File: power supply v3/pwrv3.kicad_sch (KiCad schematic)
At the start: 55 parts, among them IC1 TLV3701IDBVR, IC2 LM25145RGYR, IC3 LMR50410YQDBVRQ1, J1 1.5 mm, J3 1933189, J4 Conn_01x04_Pin 1.27mm, Q1 35A, 30V, Q2 35A Id, 30V Vds

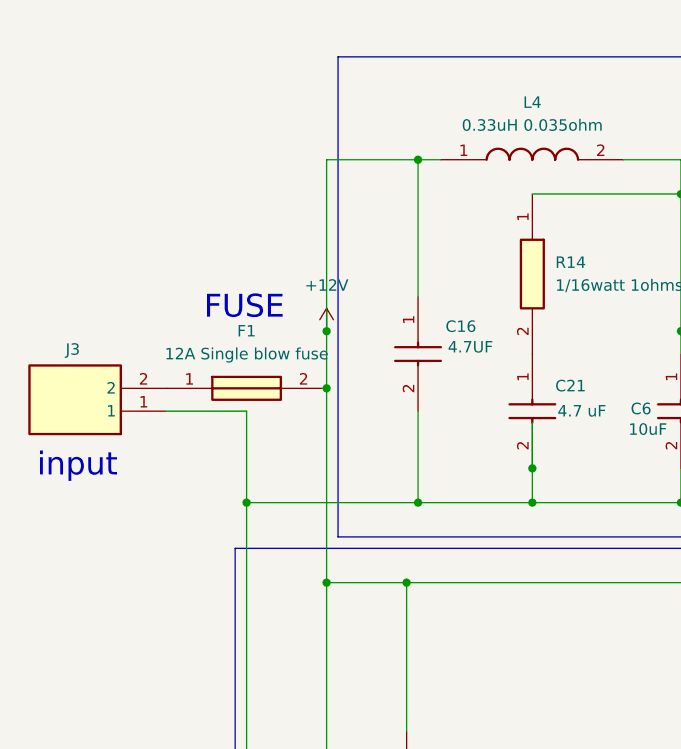
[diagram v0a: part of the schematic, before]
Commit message: board joe v2 finish
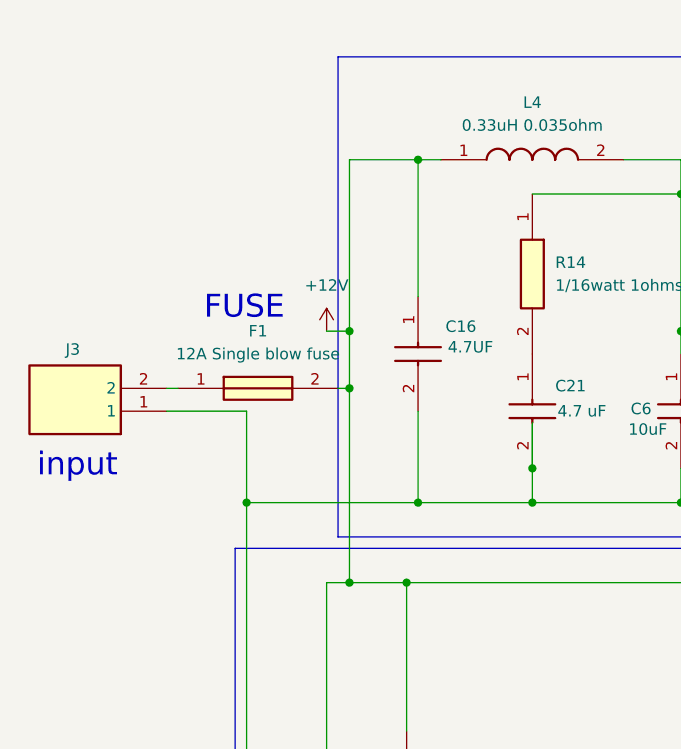
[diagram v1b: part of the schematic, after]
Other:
- moved on the sheet: F1
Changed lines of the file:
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@@
 	)
 	(junction
+		(at 48.26 72.39)
+		(diameter 0)
+		(color 0 0 0 0)
+	)
+	(junction
 		(at 68.58 59.69)
 		(diameter 0)
@@
 	)
 	(junction
-		(at 45.72 72.39)
-		(diameter 0)
-		(color 0 0 0 0)
-	)
-	(junction
 		(at 269.24 41.91)
 		(diameter 0)
@@
 	)
 	(junction
-		(at 45.72 50.8)
+		(at 222.25 129.54)
 		(diameter 0)
 		(color 0 0 0 0)
 	)
 	(junction
-		(at 222.25 129.54)
+		(at 54.61 72.39)
 		(diameter 0)
 		(color 0 0 0 0)
 	)
 	(junction
-		(at 54.61 72.39)
+		(at 48.26 50.8)
 		(diameter 0)
 		(color 0 0 0 0)
 	)
 	(junction
-		(at 96.52 123.19)
+		(at 48.26 44.45)
 		(diameter 0)
 		(color 0 0 0 0)
 	)
 	(junction
-		(at 234.95 21.59)
+		(at 96.52 123.19)
 		(diameter 0)
 		(color 0 0 0 0)
 	)
 	(junction
-		(at 260.35 41.91)
+		(at 234.95 21.59)
 		(diameter 0)
 		(color 0 0 0 0)
 	)
 	(junction
-		(at 45.72 44.45)
+		(at 260.35 41.91)
 		(diameter 0)
 		(color 0 0 0 0)
@@
 	(wire
 		(pts
-			(xy 45.72 72.39) (xy 54.61 72.39)
-		)
-		(stroke
-			(width 0)
-			(type default)
-		)
-	)
-	(wire
-		(pts
 			(xy 54.61 163.83) (xy 54.61 133.35)
 		)
@@
 	(wire
 		(pts
+			(xy 48.26 72.39) (xy 54.61 72.39)
+		)
+		(stroke
+			(width 0)
+			(type default)
+		)
+	)
+	(wire
+		(pts
 			(xy 118.11 50.8) (xy 132.08 50.8)
 		)
@@
 	(wire
 		(pts
-			(xy 45.72 25.4) (xy 45.72 44.45)
+			(xy 48.26 25.4) (xy 48.26 44.45)
 		)
 		(stroke
@@
 	(wire
 		(pts
-			(xy 45.72 44.45) (xy 45.72 50.8)
+			(xy 48.26 44.45) (xy 48.26 50.8)
 		)
 		(stroke
@@
 	(wire
 		(pts
+			(xy 27.94 50.8) (xy 29.21 50.8)
+		)
+		(stroke
+			(width 0)
+			(type default)
+		)
+	)
+	(wire
+		(pts
 			(xy 161.29 116.84) (xy 175.26 116.84)
 		)
@@
 	(wire
 		(pts
-			(xy 45.72 25.4) (xy 55.88 25.4)
+			(xy 48.26 72.39) (xy 45.72 72.39)
+		)
+		(stroke
+			(width 0)
+			(type default)
+		)
+	)
+	(wire
+		(pts
+			(xy 48.26 25.4) (xy 55.88 25.4)
 		)
 		(stroke
@@
 	(wire
 		(pts
+			(xy 48.26 44.45) (xy 45.72 44.45)
+		)
+		(stroke
+			(width 0)
+			(type default)
+		)
+	)
+	(wire
+		(pts
 			(xy 228.6 34.29) (xy 232.41 34.29)
 		)
@@
 	(wire
 		(pts
+			(xy 46.99 50.8) (xy 48.26 50.8)
+		)
+		(stroke
+			(width 0)
+			(type default)
+		)
+	)
+	(wire
+		(pts
 			(xy 205.74 144.78) (xy 205.74 139.7)
 		)
@@
 	(wire
 		(pts
-			(xy 45.72 50.8) (xy 45.72 72.39)
+			(xy 48.26 50.8) (xy 48.26 72.39)
 		)
 		(stroke
@@
 	(symbol
 		(lib_id "SF-1206HH12M-2:SF-1206HH12M-2")
-		(at 27.94 50.8 0)
+		(at 29.21 50.8 0)
 		(unit 1)
 		(exclude_from_sim no)
@@
 		(dnp no)
 		(property "Reference" "F1"
-			(at 36.83 44.45 0)
+			(at 38.1 44.45 0)
 			(effects
 				(font
@@
 		)
 		(property "Value" "SF-1206HH12M-2"
-			(at 36.83 46.99 0)
+			(at 38.1 46.99 0)
 			(effects
 				(font
@@
 		)
 		(property "Footprint" "Fuse:Fuse_1206_3216Metric"
-			(at 41.91 146.99 0)
+			(at 43.18 146.99 0)
 			(effects
 				(font
@@
 		)
 		(property "Datasheet" "https://www.bourns.com/docs/product-datasheets/sf-1206hh-m.pdf?sfvrsn=349c72f6_12"
-			(at 41.91 246.99 0)
+			(at 43.18 246.99 0)
 			(effects
 				(font
@@
 		)
 		(property "Description" "Surface Mount Fuses 12A Single blow fuse 1206 SinglFuse"
-			(at 27.94 50.8 0)
+			(at 29.21 50.8 0)
 			(effects
 				(font
@@
 		)
 		(property "Height" "1.17"
-			(at 41.91 446.99 0)
+			(at 43.18 446.99 0)
 			(effects
 				(font
@@
 		)
 		(property "Mouser Part Number" "652-SF-1206HH12M-2"
-			(at 41.91 546.99 0)
+			(at 43.18 546.99 0)
 			(effects
 				(font
@@
 		)
 		(property "Mouser Price/Stock" "https://www.mouser.co.uk/ProductDetail/Bourns/SF-1206HH12M-2?qs=gTYE2QTfZfTw6Z9W9invMQ%3D%3D"
-			(at 41.91 646.99 0)
+			(at 43.18 646.99 0)
 			(effects
 				(font
@@
 		)
 		(property "Manufacturer_Name" "Bourns"
-			(at 41.91 746.99 0)
+			(at 43.18 746.99 0)
 			(effects
 				(font
@@
 		)
 		(property "Manufacturer_Part_Number" "SF-1206HH12M-2"
-			(at 41.91 846.99 0)
+			(at 43.18 846.99 0)
 			(effects
 				(font
@@
 		)
 		(property "Field10" "12A Single blow fuse"
-			(at 36.83 46.99 0)
+			(at 38.1 46.99 0)
 			(effects
 				(font
